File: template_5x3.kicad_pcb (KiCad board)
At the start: 2 copper layers, 118.1 x 55.1 mm, 15 parts, among them P1 PWR_JACK_2.5x5.5, P2 HEADER_01X03_SMD_RA, P3 HEADER_01X03_SMD_RA, P4 HEADER_01X03_SMD_RA, P5 HEADER_01X03_SMD_RA, P6 HEADER_01X02_SMD_RA, P7 BNC_DOUBLE_RA, SW1 SPST_SLIDE_AS

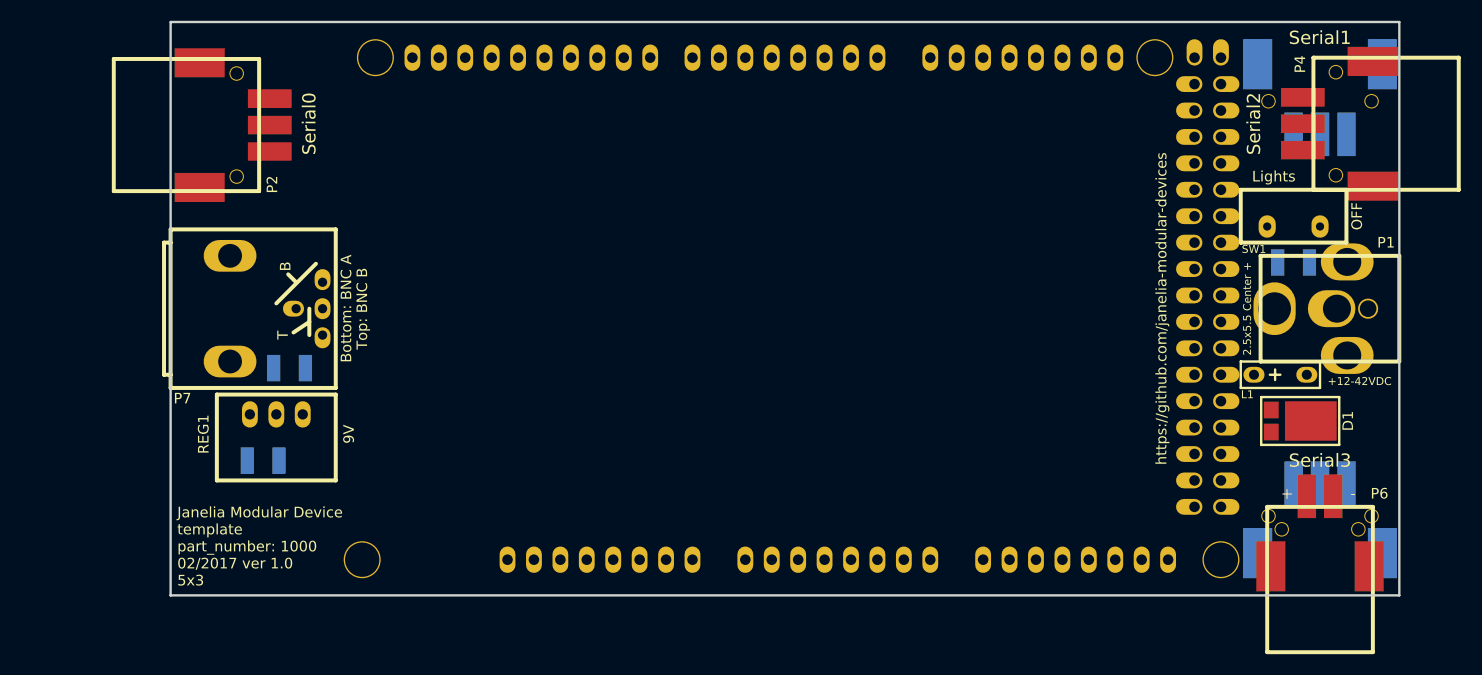
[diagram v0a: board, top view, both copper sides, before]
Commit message: Starting from scratch.
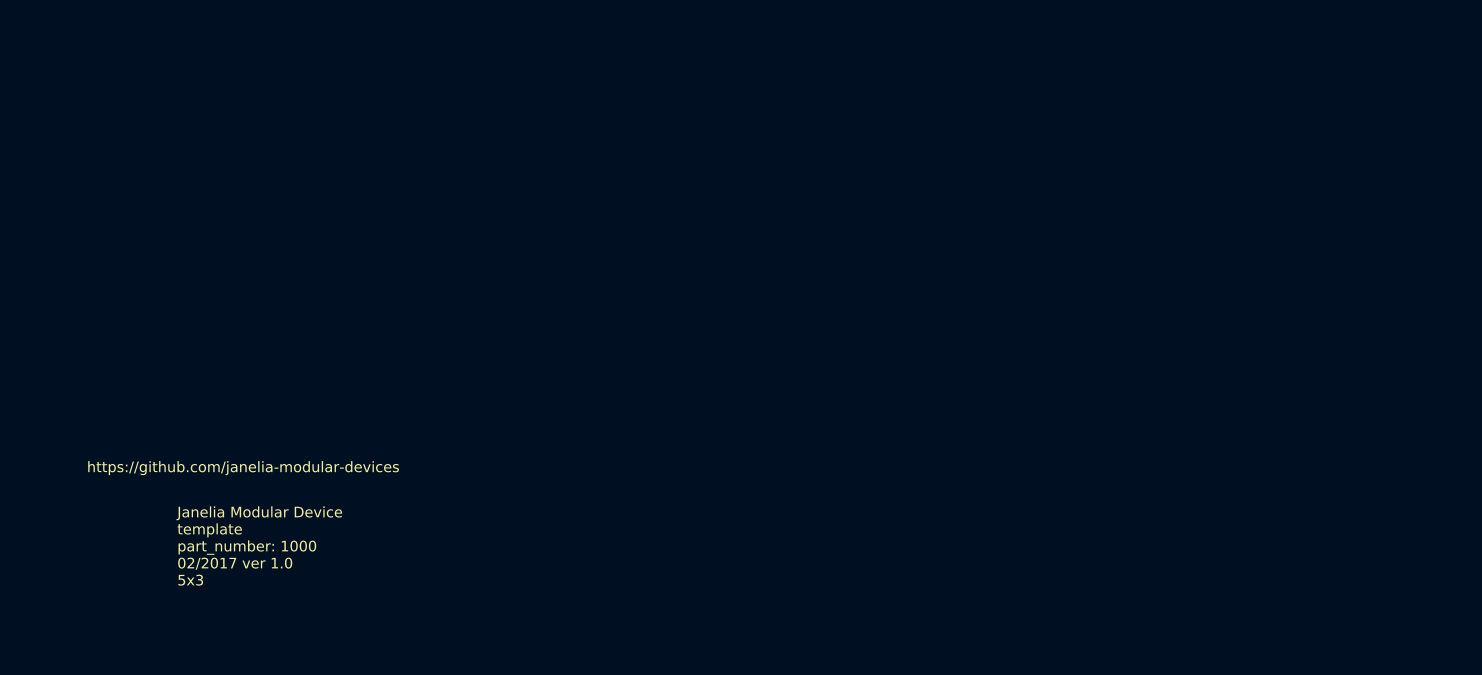
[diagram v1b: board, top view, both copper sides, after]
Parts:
- removed ARDUINO1: ARDUINO_MEGA, template_5x3:ARDUINO_MEGA_SHIELD
- removed C1, C2, C3: 10uF, template_5x3:SM1210
- removed D1: diode_schottky_45V_10A, template_5x3:CFP15
- removed L1: LED_24V, template_5x3:LED_555-3XXX
- removed P1: PWR_JACK_2.5x5.5, template_5x3:DCJACK_2PIN_HIGHCURRENT
- removed P2, P3, P4, P5: HEADER_01X03_SMD_RA, template_5x3:Header_3_Pin_SMD_RA
- removed P6: HEADER_01X02_SMD_RA, template_5x3:Header_2_Pin_SMD_RA
- removed P7: BNC_DOUBLE_RA, template_5x3:BNC_DOUBLE
- removed REG1: CONV_DC_DC_9V_1A, template_5x3:DC_DC_CONV_R78C
- removed SW1: SPST_SLIDE_AS, template_5x3:SPST_SLIDE_AS
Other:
- board outline removed
- board text removed: "+"
- board text removed: "+12-42VDC"
- board text removed: "-"
- board text removed: "2.5x5.5 Center +"
- board text removed: "9V"
- board text removed: "Lights"
- board text removed: "Serial0"
- board text removed: "Serial1"
- board text removed: "Serial2"
- board text removed: "Serial3"
